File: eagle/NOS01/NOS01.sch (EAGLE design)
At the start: 38 parts, among them IC1 TL072P, IC2 TL072P, T1 2SC1815, T2 2SC1815

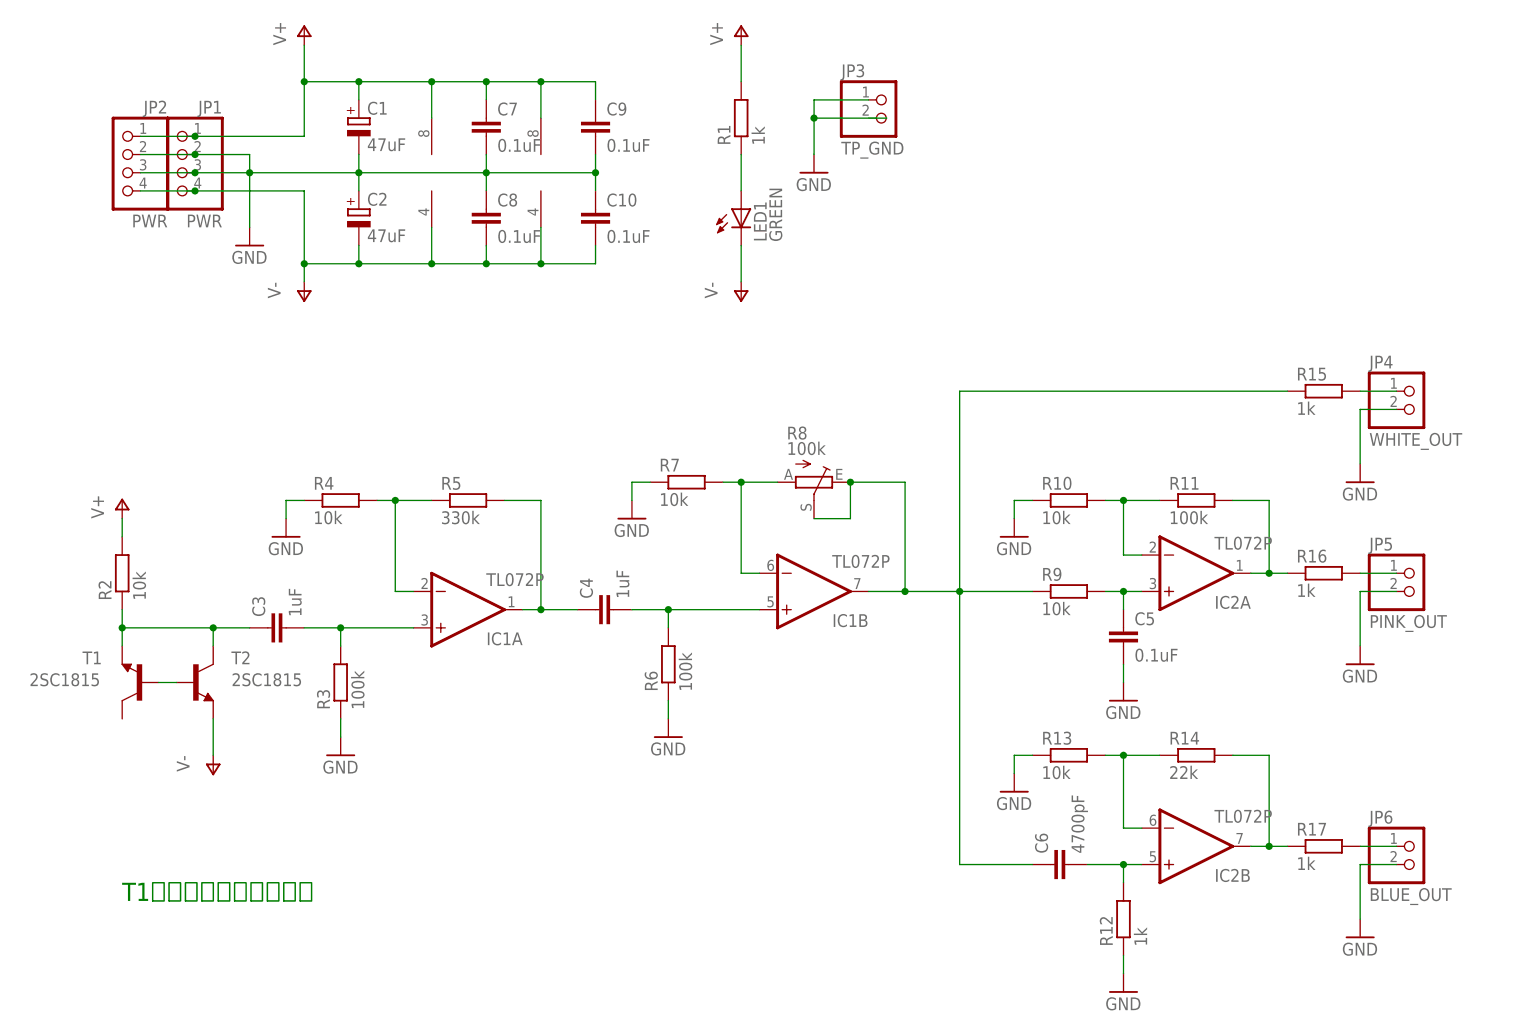
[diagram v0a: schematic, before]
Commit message: add a board design
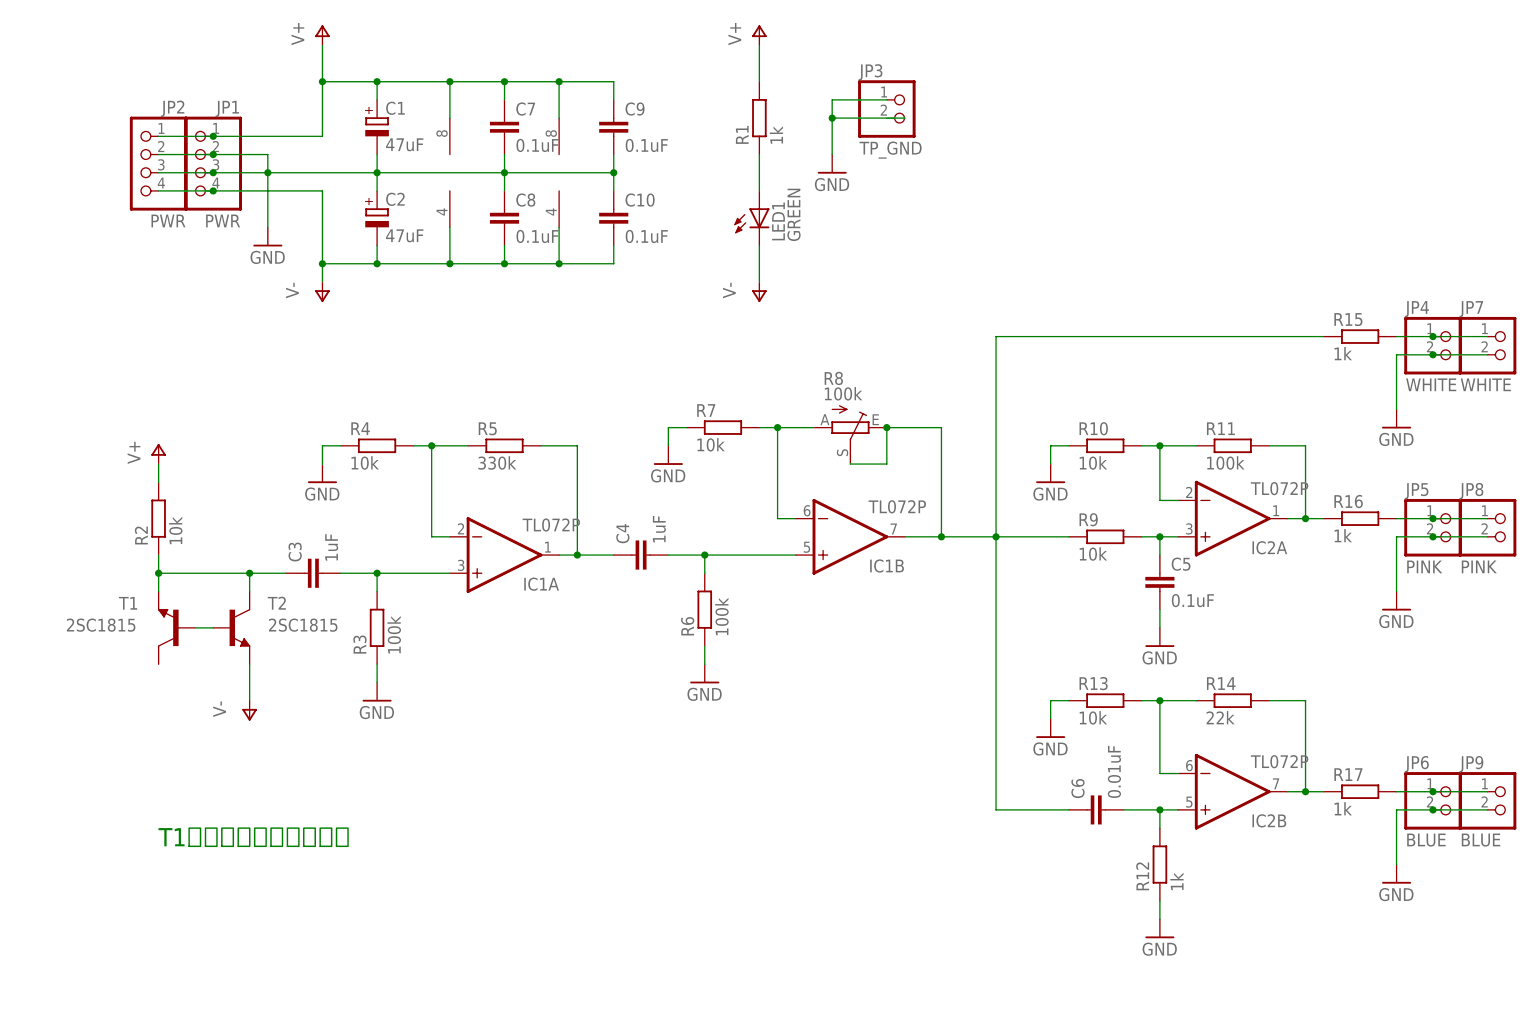
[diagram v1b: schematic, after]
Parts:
- added JP7: WHITE, pinhead:PINHD-1X2
- added JP8: PINK, pinhead:PINHD-1X2
- added JP9: BLUE, pinhead:PINHD-1X2
- C5: device rcl:C-EU050-045X075 -> rcl:C-EU075-052X106
- C6: value 4700pF -> 0.01uF
- JP4: value WHITE_OUT -> WHITE
- JP5: value PINK_OUT -> PINK
- JP6: value BLUE_OUT -> BLUE
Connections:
- removed net N$20: JP5.1, R16.2
- new net N$12: JP5.1, JP8.1, R16.2
- net GND: now also JP7.2, JP8.2, JP9.2
- net N$18: now also JP7.1
- net N$21: now also JP9.1
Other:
- moved on the sheet: C1, C10, C2, C3, C4, C5, C6, C7, C8, C9, IC1A, IC1B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
